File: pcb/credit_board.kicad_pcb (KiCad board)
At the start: 2 copper layers, 45.7 x 41.9 mm, 17 parts, among them J1 amp or pull-up, J2 amp or pull-up, J3 Jack-DC, J4 amp or pull-up, J5 clk, J6 clk, U1 74HC04, Y1 10MHz, Y2 32.768 kHz

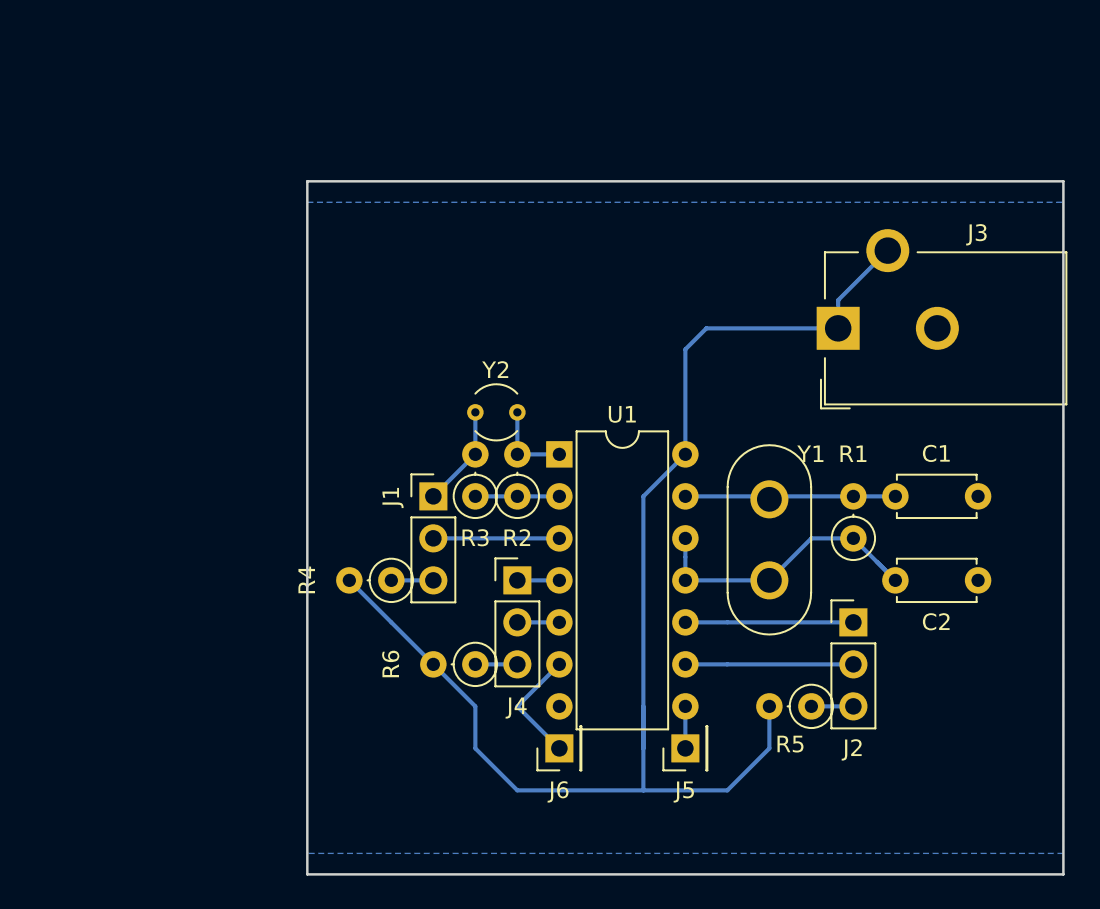
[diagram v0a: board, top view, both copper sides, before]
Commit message: board の clock 部は完成。
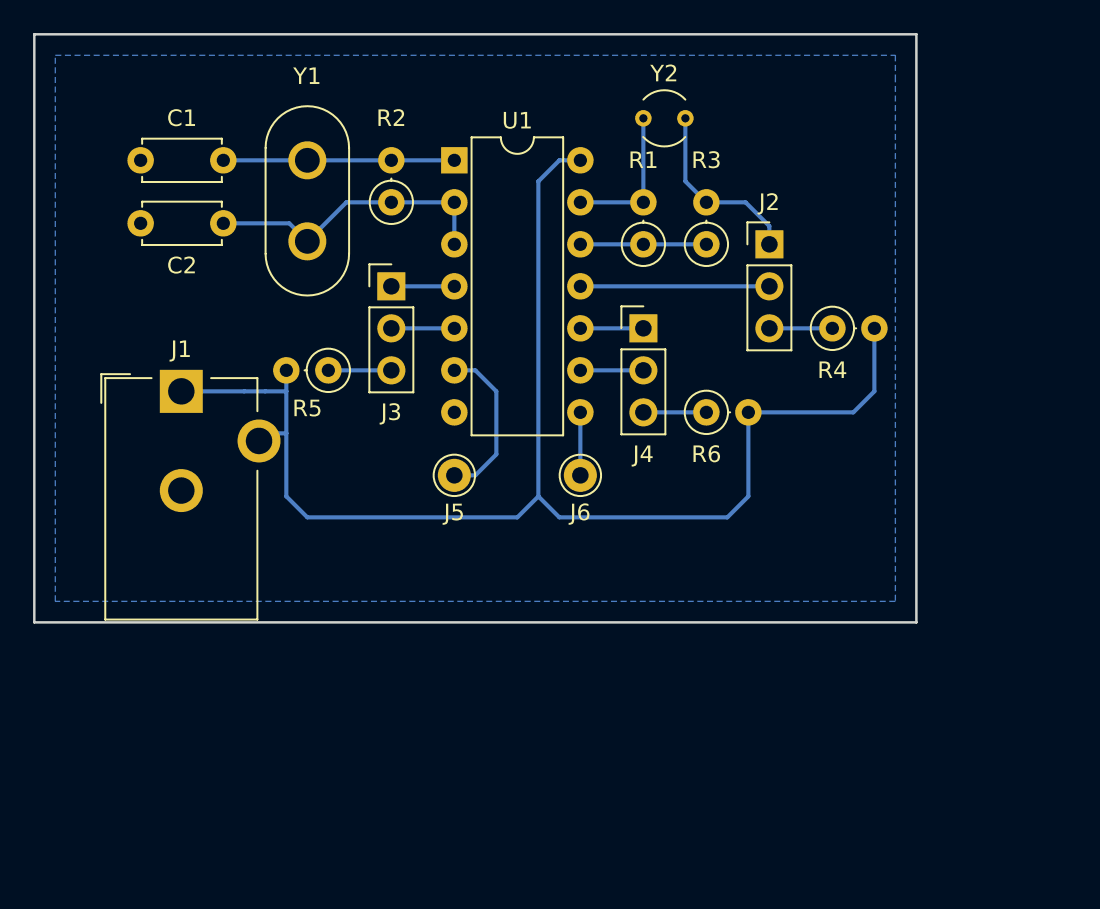
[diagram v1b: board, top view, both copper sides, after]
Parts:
- J1: value amp or pull-up -> Jack-DC; footprint Pin_Headers:Pin_Header_Straight_1x03_Pitch2.54mm -> Connectors:Barrel_Jack_CUI_PJ-102AH
- J3: value Jack-DC -> amp or pull-up; footprint Connectors:Barrel_Jack_CUI_PJ-102AH -> Pin_Headers:Pin_Header_Straight_1x03_Pitch2.54mm
- J5, J6: footprint Pin_Headers:Pin_Header_Straight_1x01_Pitch2.54mm -> Connectors:Pin_d1.0mm_L10.0mm
- R1: value 1MΩ -> 10MΩ
- R2: value 10MΩ -> 1MΩ
- moved C2 46.0 mm to (134.6, 99.1), turned to 180 degrees
- moved C1 45.4 mm to (134.6, 95.2), turned to 180 degrees
- moved R5 35.6 mm to (141.0, 108.0)
- moved Y1 34.7 mm to (139.7, 95.2)
- moved R4 30.7 mm to (171.4, 105.4), turned to 0 degrees
- moved J3 27.1 mm to (144.8, 102.9), turned to 0 degrees
- moved J2 23.4 mm to (167.6, 100.3)
- moved R1 21.8 mm to (160.0, 100.3)
- moved J5 21.6 mm to (148.6, 114.3), turned to 0 degrees
- moved R6 20.7 mm to (163.8, 110.5), turned to 0 degrees
- moved R3 20.7 mm to (163.8, 100.3)
- moved Y2 19.3 mm to (160.0, 92.7), turned to 0 degrees
- moved R2 19.3 mm to (144.8, 97.8)
- moved U1 18.9 mm to (148.6, 95.2)
- moved J4 17.0 mm to (160.0, 105.4)
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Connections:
- net Net-(J4-Pad3) renamed /pull-up2
- J1 pad 1: Net-(J1-Pad1) -> VCC
- J1 pad 2: Net-(J1-Pad2) -> GND
- J1 pad 3: Net-(J1-Pad3) -> VCC
- J2 pad 1: Net-(J2-Pad1) -> /output1
- J2 pad 2: Net-(J2-Pad2) -> /amp1
- J2 pad 3: Net-(J2-Pad3) -> /pull-up1
- J3 pad 1: VCC -> /amp3
- J3 pad 2: GND -> Net-(J3-Pad2)
- J3 pad 3: VCC -> /pull-up3
- J4 pad 1: Net-(J4-Pad1) -> /amp2
- J5 pad 1: Net-(J5-Pad1) -> /output3
- J6 pad 1: Net-(J6-Pad1) -> /output2
- R1 pad 1: Net-(C2-Pad1) -> Net-(R1-Pad1)
- R1 pad 2: Net-(C1-Pad1) -> Net-(R1-Pad2)
- R2 pad 1: Net-(R2-Pad1) -> Net-(C2-Pad1)
- R2 pad 2: Net-(R2-Pad2) -> Net-(C1-Pad1)
- R3 pad 1: Net-(R2-Pad1) -> Net-(R1-Pad1)
- R3 pad 2: Net-(J1-Pad1) -> /output1
- R4 pad 1: Net-(J1-Pad3) -> /pull-up1
- R5 pad 1: Net-(J2-Pad3) -> /pull-up3
- U1 pad 1: Net-(R2-Pad2) -> Net-(C1-Pad1)
- U1 pad 10: Net-(J2-Pad1) -> /amp2
- U1 pad 11: Net-(C2-Pad1) -> /amp1
- U1 pad 12: Net-(C2-Pad1) -> Net-(R1-Pad1)
- U1 pad 13: Net-(C1-Pad1) -> Net-(R1-Pad2)
- U1 pad 2: Net-(R2-Pad1) -> Net-(C2-Pad1)
- U1 pad 3: Net-(J1-Pad2) -> Net-(C2-Pad1)
- U1 pad 4: Net-(J4-Pad1) -> /amp3
- U1 pad 5: Net-(J4-Pad2) -> Net-(J3-Pad2)
- U1 pad 6: Net-(J6-Pad1) -> /output3
- U1 pad 8: Net-(J5-Pad1) -> /output2
- U1 pad 9: Net-(J2-Pad2) -> Net-(J4-Pad2)
- Y2 pad 1: Net-(R2-Pad2) -> Net-(R1-Pad2)
- Y2 pad 2: Net-(J1-Pad1) -> /output1
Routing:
- net /amp1: track 0.00 -> 11.4 mm
- net /output1: track 0.00 -> 11.1 mm
- net Net-(J2-Pad2): track 10.2 -> 0.00 mm
- net Net-(J2-Pad1): track 10.2 -> 0.00 mm
- net /output3: track 0.00 -> 9.94 mm
- net Net-(R1-Pad2): track 0.00 -> 8.89 mm
- net Net-(R1-Pad1): track 0.00 -> 7.62 mm
- net Net-(J1-Pad2): track 7.62 -> 0.00 mm
- net Net-(J6-Pad1): track 7.18 -> 0.00 mm
- net Net-(J1-Pad1): track 6.13 -> 0.00 mm
- net Net-(R2-Pad2): track 5.08 -> 0.00 mm
- net Net-(R2-Pad1): track 5.08 -> 0.00 mm
- net Net-(J3-Pad2): track 0.00 -> 3.81 mm
- net /pull-up3: track 0.00 -> 3.81 mm
- net /pull-up1: track 0.00 -> 3.81 mm
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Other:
- board size 45.7 x 41.9 mm -> 53.3 x 35.6 mm
